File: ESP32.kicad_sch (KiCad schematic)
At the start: 34 parts, among them IC1 L6981C50DR, IC2 L6981C33DR, J1 USB_B_Micro, J2 BATT, J3 PMS7003 Connector, J5 UART, Q1 AO3400A, SW1 RESET, SW2 BOOTSEL, U1 ESP32-C3-MINI-1

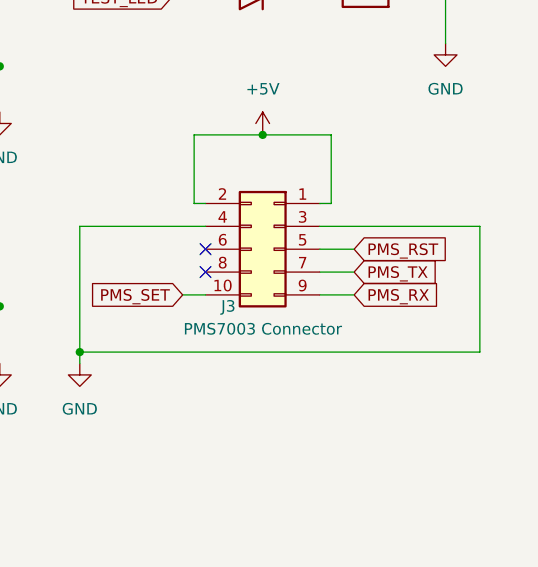
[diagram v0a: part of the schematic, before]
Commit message: Schematic + Layout
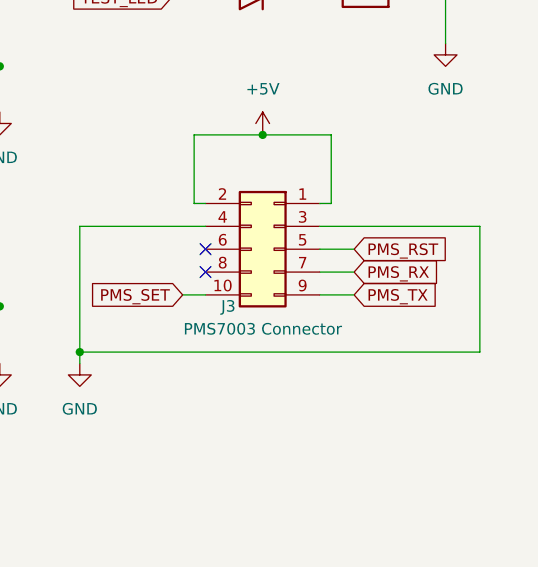
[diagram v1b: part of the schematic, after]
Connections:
- net PMS_RX: now also J3.7 (Pin_7); no longer J3.9 (Pin_9)
- net PMS_TX: now also J3.9 (Pin_9); no longer J3.7 (Pin_7)
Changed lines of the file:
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@@
+    (stroke (width 0) (type default))
+  )
+  (wire (pts (xy 261.62 147.32) (xy 265.43 147.32))
     (stroke (width 0) (type default))
   )
@@
     (stroke (width 0) (type default))
   )
-  (wire (pts (xy 261.62 147.32) (xy 265.43 147.32))
-    (stroke (width 0) (type default))
-  )
   (wire (pts (xy 71.12 132.08) (xy 74.93 132.08))
     (stroke (width 0) (type default))
@@
     (stroke (width 0) (type default))
   )
+  (wire (pts (xy 261.62 144.78) (xy 265.43 144.78))
+    (stroke (width 0) (type default))
+  )
   (wire (pts (xy 257.81 114.3) (xy 262.89 114.3))
     (stroke (width 0) (type default))
@@
   )
   (wire (pts (xy 30.48 83.82) (xy 30.48 81.28))
-    (stroke (width 0) (type default))
-  )
-  (wire (pts (xy 261.62 144.78) (xy 265.43 144.78))
     (stroke (width 0) (type default))
   )
@@
     )
   )
-  (global_label "PMS_RX" (shape input) (at 265.43 147.32 0) (fields_autoplaced)
-    (effects (font (size 1.27 1.27)) (justify left))
-    (property "Intersheetrefs" "${INTERSHEET_REFS}" (at 275.2212 147.2406 0)
+  (global_label "PMS_RX" (shape input) (at 265.43 144.78 0) (fields_autoplaced)
+    (effects (font (size 1.27 1.27)) (justify left))
+    (property "Intersheetrefs" "${INTERSHEET_REFS}" (at 275.2212 144.7006 0)
       (effects (font (size 1.27 1.27)) (justify left) hide)
     )
@@
     )
   )
-  (global_label "PMS_TX" (shape input) (at 265.43 144.78 0) (fields_autoplaced)
-    (effects (font (size 1.27 1.27)) (justify left))
-    (property "Intersheetrefs" "${INTERSHEET_REFS}" (at 274.9188 144.7006 0)
-      (effects (font (size 1.27 1.27)) (justify left) hide)
-    )
+  (global_label "PMS_TX" (shape input) (at 265.43 147.32 0) (fields_autoplaced)
+    (effects (font (size 1.27 1.27)) (justify left))
+    (property "Intersheetrefs" "${INTERSHEET_REFS}" (at 274.9188 147.2406 0)
+      (effects (font (size 1.27 1.27)) (justify left) hide)
+    )
